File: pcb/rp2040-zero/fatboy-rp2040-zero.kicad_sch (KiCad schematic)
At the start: 76 parts, among them SW1 SW_Push, U1 rp2040-zero

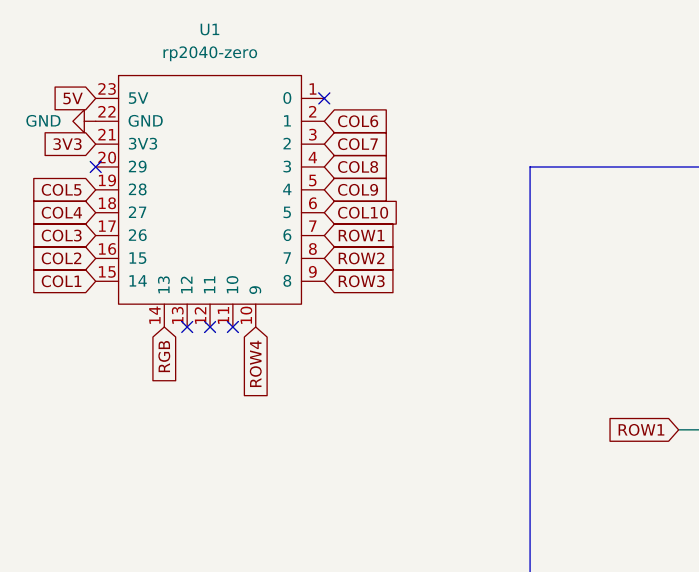
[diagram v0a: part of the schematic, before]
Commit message: reposition rows
Signed-off-by: Anant Thazhemadam <anant.thazhemadam@gmail.com>
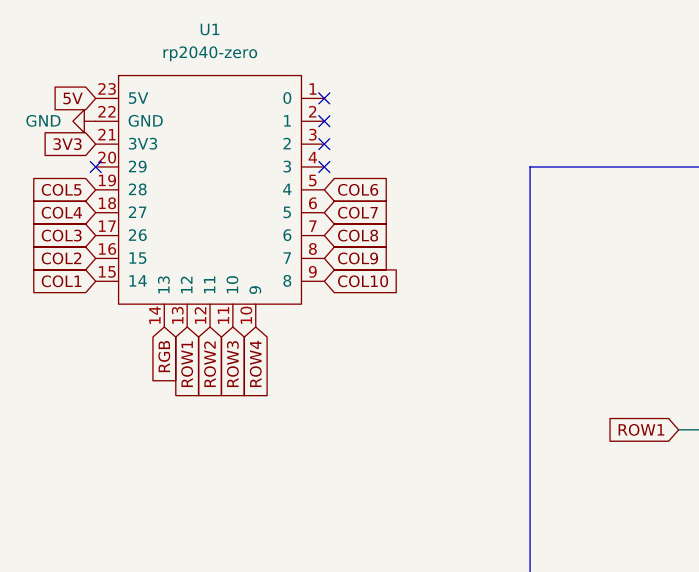
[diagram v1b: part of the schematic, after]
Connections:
- net COL10: now also U1.9 (8); no longer U1.6 (5)
- net COL6: now also U1.5 (4); no longer U1.2 (1)
- net COL7: now also U1.6 (5); no longer U1.3 (2)
- net COL8: now also U1.7 (6); no longer U1.4 (3)
- net COL9: now also U1.8 (7); no longer U1.5 (4)
- net ROW1: now also U1.13 (12); no longer U1.7 (6)
- net ROW2: now also U1.12 (11); no longer U1.8 (7)
- net ROW3: now also U1.11 (10); no longer U1.9 (8)
